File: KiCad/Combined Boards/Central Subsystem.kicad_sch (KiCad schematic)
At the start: 42 parts, among them J1 Antenna, J2 GPIO, J3 Debug, J4 Signal debug, J7 STEMMA QT, J9 Power, Q1 SI2301CDS-T1-GE3, SW1 Power, U2 STM32WLE5CCU6, Y1 32 MHz

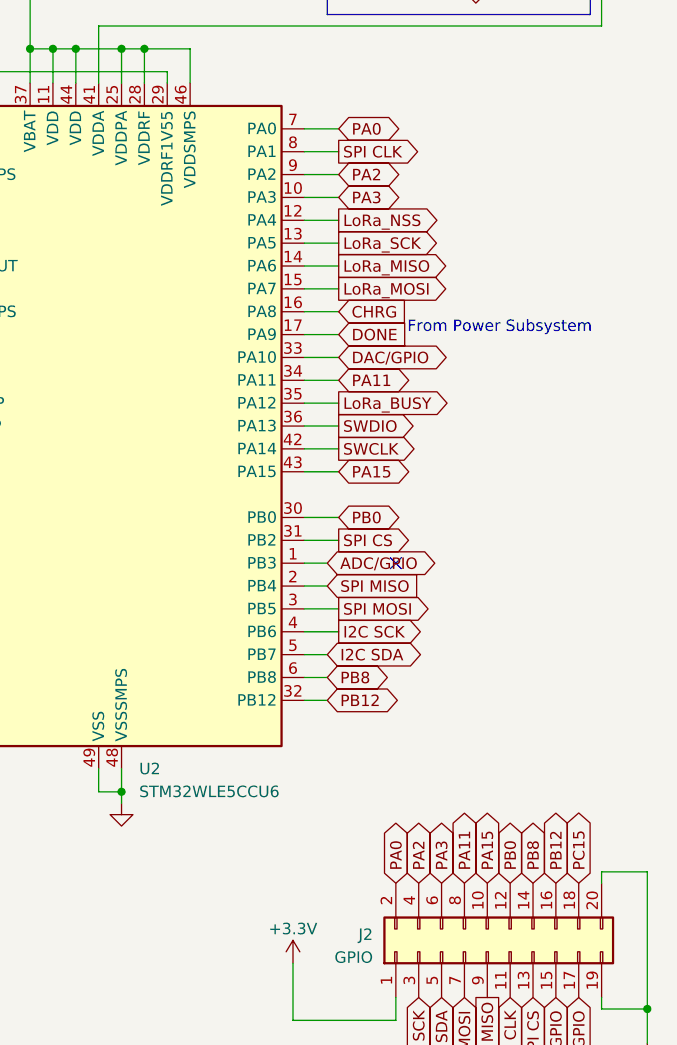
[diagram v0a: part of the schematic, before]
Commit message: Include UART pins
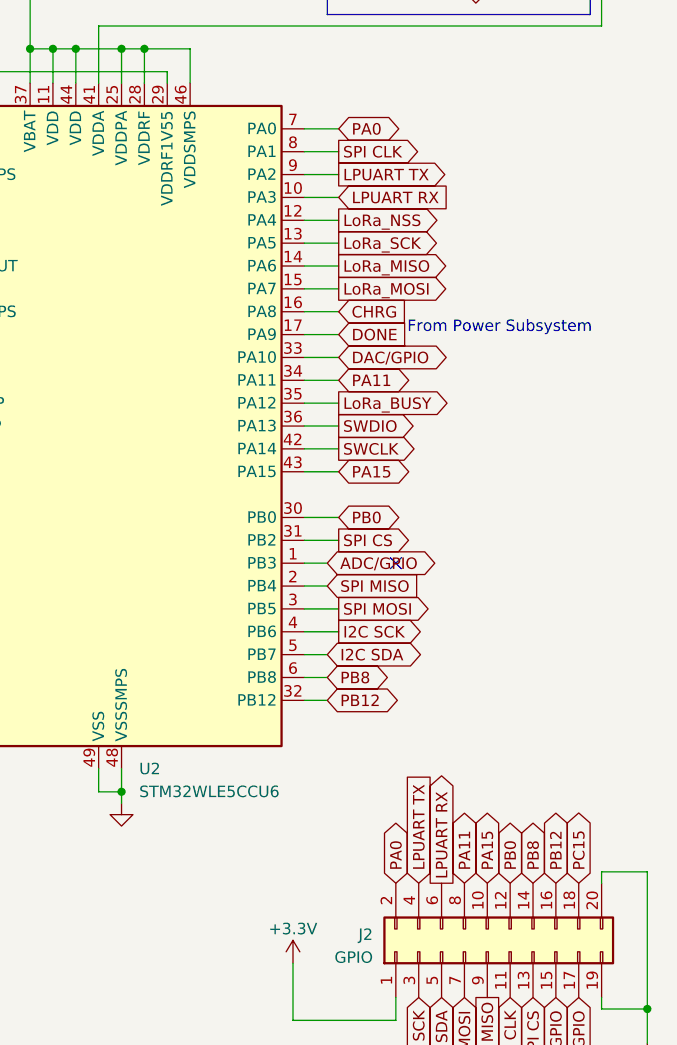
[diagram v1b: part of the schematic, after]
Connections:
- net PA2 renamed  LPUART TX
- net  LPUART TX: no longer J2.4 (Pin_4)
- net PA3 renamed LPUART RX
- new net LPUART TX: J2.4 (Pin_4)
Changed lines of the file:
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@@
     )
   )
-  (global_label "PA3" (shape bidirectional) (at 223.52 68.58 0) (fields_autoplaced)
+  (global_label "LPUART RX" (shape input) (at 223.52 68.58 0) (fields_autoplaced)
     (effects (font (size 1.27 1.27)) (justify left))
-    (property "Intersheetrefs" "${INTERSHEET_REFS}" (at 231.1052 68.58 0)
+    (property "Intersheetrefs" "${INTERSHEET_REFS}" (at 236.8277 68.58 0)
       (effects (font (size 1.27 1.27)) (justify left) hide)
     )
@@
     )
   )
-  (global_label "PA3" (shape bidirectional) (at 234.95 144.78 90) (fields_autoplaced)
+  (global_label "LPUART RX" (shape output) (at 234.95 144.78 90) (fields_autoplaced)
     (effects (font (size 1.27 1.27)) (justify left))
-    (property "Intersheetrefs" "${INTERSHEET_REFS}" (at 234.95 137.1948 90)
+    (property "Intersheetrefs" "${INTERSHEET_REFS}" (at 234.95 131.4723 90)
       (effects (font (size 1.27 1.27)) (justify left) hide)
     )
@@
     )
   )
-  (global_label "PA2" (shape bidirectional) (at 232.41 144.78 90) (fields_autoplaced)
+  (global_label "LPUART TX" (shape input) (at 232.41 144.78 90) (fields_autoplaced)
     (effects (font (size 1.27 1.27)) (justify left))
-    (property "Intersheetrefs" "${INTERSHEET_REFS}" (at 232.41 137.1948 90)
+    (property "Intersheetrefs" "${INTERSHEET_REFS}" (at 232.41 131.7747 90)
       (effects (font (size 1.27 1.27)) (justify left) hide)
     )
@@
     )
   )
-  (global_label "PA2" (shape bidirectional) (at 223.52 66.04 0) (fields_autoplaced)
+  (global_label " LPUART TX" (shape output) (at 223.52 66.04 0) (fields_autoplaced)
     (effects (font (size 1.27 1.27)) (justify left))
-    (property "Intersheetrefs" "${INTERSHEET_REFS}" (at 231.1052 66.04 0)
+    (property "Intersheetrefs" "${INTERSHEET_REFS}" (at 237.4929 66.04 0)
       (effects (font (size 1.27 1.27)) (justify left) hide)
     )
